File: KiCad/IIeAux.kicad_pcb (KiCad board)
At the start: 4 copper layers, 99.7 x 77.5 mm, 22 parts, among them J1 Aux Slot, J2 Double Hi-Res, J3 PAL, U1 TangNano9K, U2 SN74LVC245AN, U3 SN74LVC245AN, U4 SN74LVC245AN, U5 SN74LVC245AN, U6 74LS374, U7 74LS245, U8 SN74LVC245AN

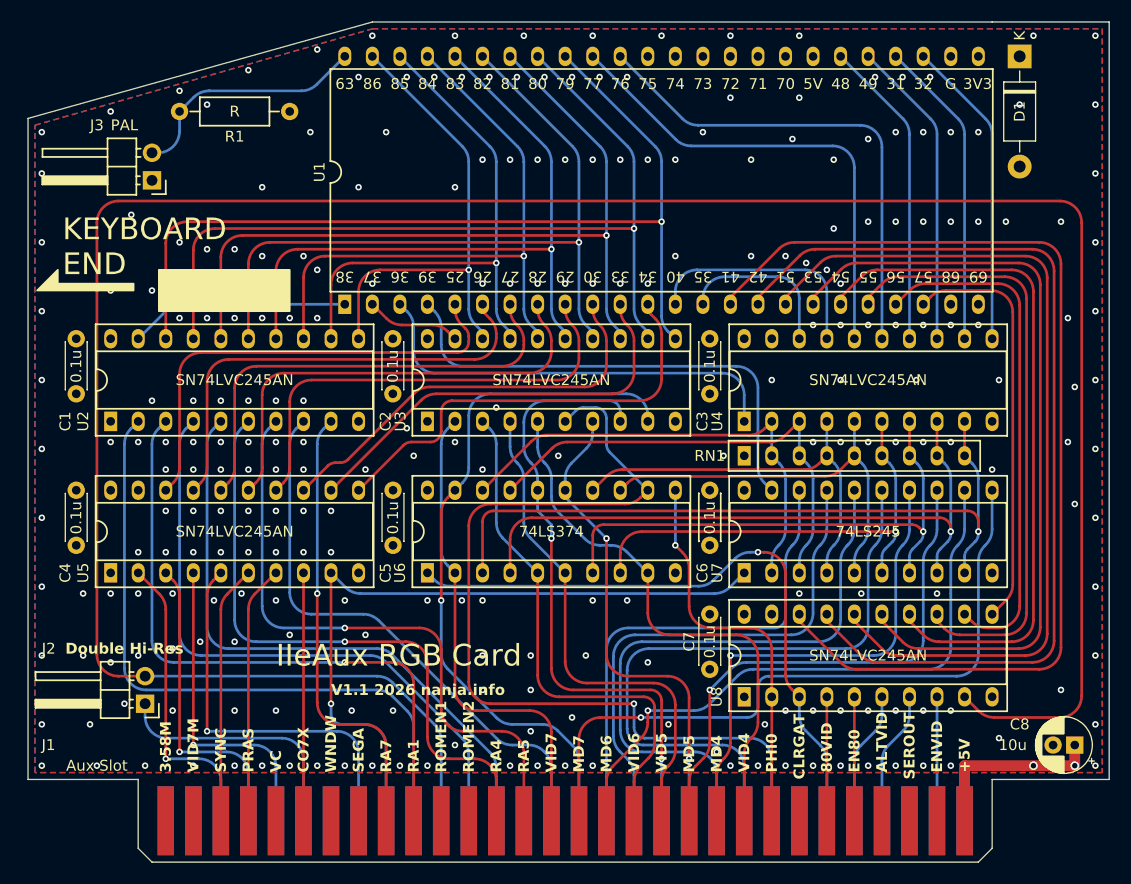
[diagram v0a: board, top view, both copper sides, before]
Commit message: V1.0 first batch
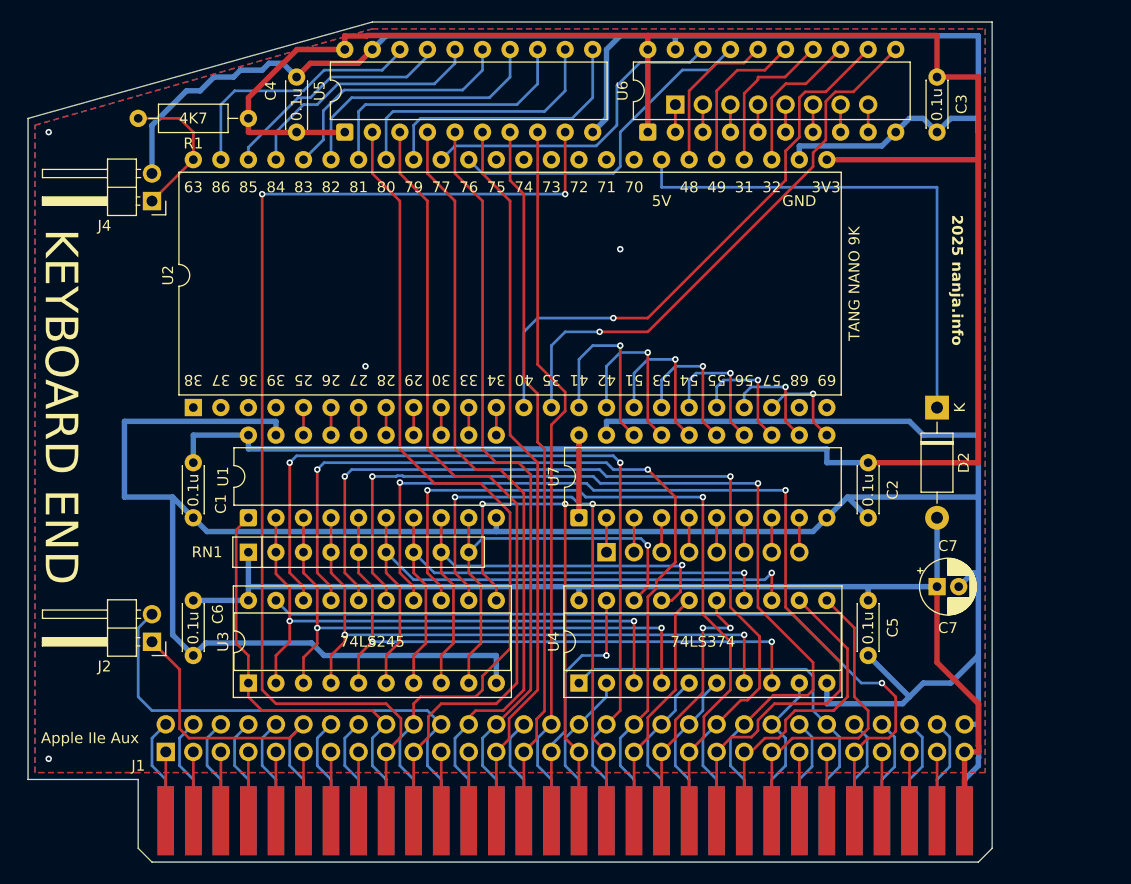
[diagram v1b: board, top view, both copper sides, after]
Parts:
- removed the C6 at (169.5, 111.8)
- removed the U2 at (114.3, 105.4)
- added J4: PAL, IIeAux:PinHeader_1x02_P2.54mm_Horizontal, F.Cu at (118.1, 85.1)
- added J5: Y, IIeAux:PinSocket_1x08_P2.54mm_Vertical, B.Cu at (160.0, 117.5)
- added J6: X, IIeAux:PinSocket_1x08_P2.54mm_Vertical, B.Cu at (166.4, 76.2)
- J1: value Aux Slot -> Apple IIe Aux
- J2: value Double Hi-Res -> Double HiRes
- J3: value PAL -> Aux; footprint IIeAux:PinHeader_1x02_P2.54mm_Horizontal -> IIeAux:PinSocket_2x30_P2.54mm; moved to B.Cu
- R1: value R -> 4K7
- U1: renamed from U5; footprint IIeAux:DIP-20_W7.62mm_Socket -> IIeAux:DIP-20_W7.62mm
- U5: renamed from U3; footprint IIeAux:DIP-20_W7.62mm_Socket -> IIeAux:DIP-20_W7.62mm
- U6: renamed from U4; footprint IIeAux:DIP-20_W7.62mm_Socket -> IIeAux:DIP-20_W7.62mm
- U7: renamed from U8; footprint IIeAux:DIP-20_W7.62mm_Socket -> IIeAux:DIP-20_W7.62mm
- moved C2 73.1 mm to (184.2, 109.2)
- moved C4 58.5 mm to (131.4, 78.7), turned to 90 degrees
- moved J3 52.7 mm to (119.4, 135.9), turned to -90 degrees
- moved C5 50.0 mm to (184.2, 121.9)
- moved U3 46.8 mm to (127.0, 129.5)
- moved RN1 46.6 mm to (127.0, 117.5)
- moved D2 33.3 mm to (190.5, 104.1)
- moved C3 32.0 mm to (190.5, 73.7)
- moved U6 28.1 mm to (163.8, 78.7)
- moved U5 27.7 mm to (135.9, 78.7)
- moved U7 22.5 mm to (157.5, 114.3)
- moved C6 21.0 mm to (121.9, 121.9)
- moved C7 19.4 mm to (190.5, 120.7), turned to 0 degrees
- moved U4 17.3 mm to (157.5, 129.5)
- moved U2 16.9 mm to (121.9, 104.1)
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- renumbered C4 to C2, C7 to C4, C2 to C5, C5 to C6, C8 to C7, D1 to D2, U1 to U2, U7 to U3, U6 to U4
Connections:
- net A0 renamed Net-(U2-IOT12B_79)
- net A1 renamed Net-(U2-IOT12A_80)
- net A2 renamed Net-(U2-IOT11B_81)
- net A3 renamed Net-(U2-IOT11A_82)
- net A4 renamed Net-(U2-IOT10B_83)
- net A5 renamed Net-(U2-IOT10A_84)
- net A6 renamed Net-(U2-IOT8B_85)
- net A7 renamed Net-(U2-IOT8A_86)
- C5 pad 1: +3V3 -> +5V
- J3 pad 1: GND -> 3.58M
- J3 pad 2: Net-(J3-Pin_2) -> VID7M
- R1 pad 2: Net-(J3-Pin_2) -> Net-(J4-Pin_1)
- U1 pad 1: +3V3 -> R/W
- U1 pad 2: GR -> D0
- U1 pad 3: RA10 -> D1
- U1 pad 4: RA9 -> D2
- U1 pad 5: Q3 -> D3
- U1 pad 6: SYNC -> D4
- U1 pad 7: PRAS -> D5
- U1 pad 8: C07X -> D6
- U1 pad 9: R/W -> D7
- U2 pad 1: RA_EN -> unconnected-(U2-38_IOB31B-Pad1)
- U2 pad 13: Net-(U1-40_IOB33B) -> Net-(U2-40_IOB33B)
- U2 pad 14: Net-(U1-35_IOB29A) -> Net-(U2-35_IOB29A)
- U2 pad 2: VID_EN -> unconnected-(U2-37_IOB31A-Pad2)
- U2 pad 27: Net-(U1-IOB15B_32) -> Net-(U2-IOB15B_32)
- U2 pad 28: Net-(U1-IOB15A_31) -> Net-(U2-IOB15A_31)
- U2 pad 29: Net-(U1-IOR24A_49) -> Net-(U2-IOR24A_49)
- U2 pad 3: D_R/W -> unconnected-(U2-36_IOB29B-Pad3)
- U2 pad 30: Net-(U1-IOR24B_48) -> Net-(U2-IOR24B_48)
- U2 pad 38: Net-(U1-IOT37B_76) -> Net-(U2-IOT37B_76)
- U2 pad 39: Net-(U1-IOT37A_77) -> Net-(U2-IOT37A_77)
- U2 pad 4: MD_EN -> unconnected-(U2-39_IOB33A-Pad4)
- U2 pad 48: Net-(J3-Pin_2) -> Net-(J4-Pin_1)
- U3 pad 19: MD_EN -> EN80
- U4 pad 12: VID3 -> VID4
- U4 pad 13: D3 -> D4
- U4 pad 14: D2 -> D5
- U4 pad 15: VID2 -> VID5
- U4 pad 16: VID1 -> VID6
- U4 pad 17: D1 -> D6
- U4 pad 18: D0 -> D7
- U4 pad 19: VID0 -> VID7
- U4 pad 2: VID7 -> VID0
- U4 pad 3: D7 -> D0
- U4 pad 4: D6 -> D1
- U4 pad 5: VID6 -> VID1
- U4 pad 6: VID5 -> VID2
- U4 pad 7: D5 -> D2
- U4 pad 8: D4 -> D3
- U4 pad 9: VID4 -> VID3
- U5 pad 19: VID_EN -> GND
- U5 pad 2: VID7 -> RA0
- U5 pad 3: VID6 -> RA1
- U5 pad 4: VID5 -> RA2
- U5 pad 5: VID4 -> RA3
- U5 pad 6: VID3 -> RA4
- U5 pad 7: VID2 -> RA5
- U5 pad 8: VID1 -> RA6
- U5 pad 9: VID0 -> RA7
- U6 pad 1: D_R/W -> +3V3
- U6 pad 11: Net-(U1-IOB15B_32) -> Net-(U2-35_IOB29A)
- U6 pad 12: Net-(U1-IOB15A_31) -> Net-(U2-40_IOB33B)
- U6 pad 13: Net-(U1-IOR24A_49) -> Net-(U2-IOB15B_32)
- U6 pad 14: Net-(U1-IOR24B_48) -> Net-(U2-IOB15A_31)
- U6 pad 15: Net-(U1-IOT37B_76) -> Net-(U2-IOR24A_49)
- U6 pad 16: Net-(U1-IOT37A_77) -> Net-(U2-IOR24B_48)
- U6 pad 17: Net-(U1-40_IOB33B) -> Net-(U2-IOT37B_76)
- U6 pad 18: Net-(U1-35_IOB29A) -> Net-(U2-IOT37A_77)
- U6 pad 2: D0 -> X0
- U6 pad 3: D1 -> X1
- U6 pad 4: D2 -> X2
- U6 pad 5: D3 -> X3
- U6 pad 6: D4 -> X4
- U6 pad 7: D5 -> X5
- U6 pad 8: D6 -> X6
- U6 pad 9: D7 -> X7
- U7 pad 2: PHI0 -> Y0
- U7 pad 3: PHI1 -> Y1
- U7 pad 4: 80VID -> Y2
- U7 pad 5: EN80 -> Y3
- U7 pad 6: R/W80 -> Y4
- U7 pad 7: LDPS -> Y5
- U7 pad 8: 14M -> Y6
- U7 pad 9: AN3 -> Y7
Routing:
- net GND: track 5.08 -> 407.6 mm, vias 252 -> 4
- net AN3: track 229.5 -> 47.1 mm
- net +3V3: track 309.9 -> 231.1 mm
- net Net-(U2-41_IOB41A): track 95.9 -> 17.6 mm, vias 0 -> 1
- net Net-(U2-42_IOB41B): track 87.7 -> 16.3 mm, vias 0 -> 1
- net VID3: track 83.8 -> 14.8 mm, vias 1 -> 0
- net Net-(U2-51_IOR17B): track 79.6 -> 15.0 mm, vias 0 -> 1
- net EN80: track 11.4 -> 75.0 mm, vias 0 -> 1
- net RA7: track 41.7 -> 103.3 mm, vias 1 -> 2
- net Net-(U2-IOT12B_79): track 85.6 -> 25.2 mm, vias 1 -> 0
- net Net-(U2-53_IOR15B): track 71.4 -> 13.7 mm, vias 0 -> 1
- net Net-(U2-IOT12A_80): track 79.3 -> 25.2 mm, vias 1 -> 0
- net Net-(U2-40_IOB33B): track 0.00 -> 53.2 mm, vias 0 -> 1
- net Net-(U2-35_IOB29A): track 0.00 -> 51.6 mm, vias 0 -> 1
- net Net-(U2-54_IOR15A): track 63.3 -> 12.8 mm, vias 0 -> 1
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- removed copper zone on In1.Cu, net GND
- removed copper zone on In2.Cu, net GND
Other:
- board size 99.7 x 77.5 mm -> 88.9 x 77.5 mm
- copper layers 4 -> 2
- board text added: "+5V"
- board text added: "14M"
- board text added: "2025 nanja.info"
- board text added: "3.58M"
- board text added: "7M"
- board text added: "80VID"
- board text added: "ALTVID"
- board text added: "AN3"
- board text added: "C07X"
- board text added: "CASEN"
- board text added: "CLRGAT"
- board text added: "EN80"
- board text added: "ENTMG"
- board text added: "ENVID"
- board text added: "FRCTXT"
- board text added: "GND"
- board text added: "GR"
- board text added: "H0"
- board text added: "LDPS"
- board text added: "MD0"
- board text added: "MD1"
- board text added: "MD2"
- board text added: "MD3"
- board text added: "MD4"
- board text added: "MD5"
- board text added: "MD6"
- board text added: "MD7"
- board text added: "PCAS"
- board text added: "PHI0"
- board text added: "PHI1"
- board text added: "PRAS"
- board text added: "R/W"
- board text added: "R/W80"
- board text added: "RA0"
- board text added: "RA1"
- board text added: "RA10"
- board text added: "RA2"
- board text added: "RA3"
- board text added: "RA4"
- board text added: "RA5"
- board text added: "RA6"
- board text added: "RA7"
- board text added: "RA9"
- board text added: "ROMEN1"
- board text added: "ROMEN2"
- board text added: "SEGA"
- board text added: "SEGB"
- board text added: "SEROUT"
- board text added: "SYNC"
- board text added: "VC"
- board text added: "VID 7M"
- board text added: "VID0"
- board text added: "VID1"
- board text added: "VID2"
- board text added: "VID3"
- board text added: "VID4"
- board text added: "VID5"
- board text added: "VID6"
- board text added: "VID7"
- board text added: "WNDW"
- board text added: "X0"
- board text added: "X1"
- board text added: "X2"
- board text added: "X3"
- board text added: "X4"
- board text added: "X5"
- board text added: "X6"
- board text added: "X7"
- board text added: "Y0"
- board text added: "Y1"
- board text added: "Y2"
- board text added: "Y3"
- board text added: "Y4"
- board text added: "Y5"
- board text added: "Y6"
- board text added: "Y7"
- board text removed: "IIeAux RGB Card"
- board text removed: "V1.1 2026 nanja.info"
